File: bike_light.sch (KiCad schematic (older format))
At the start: 0 parts

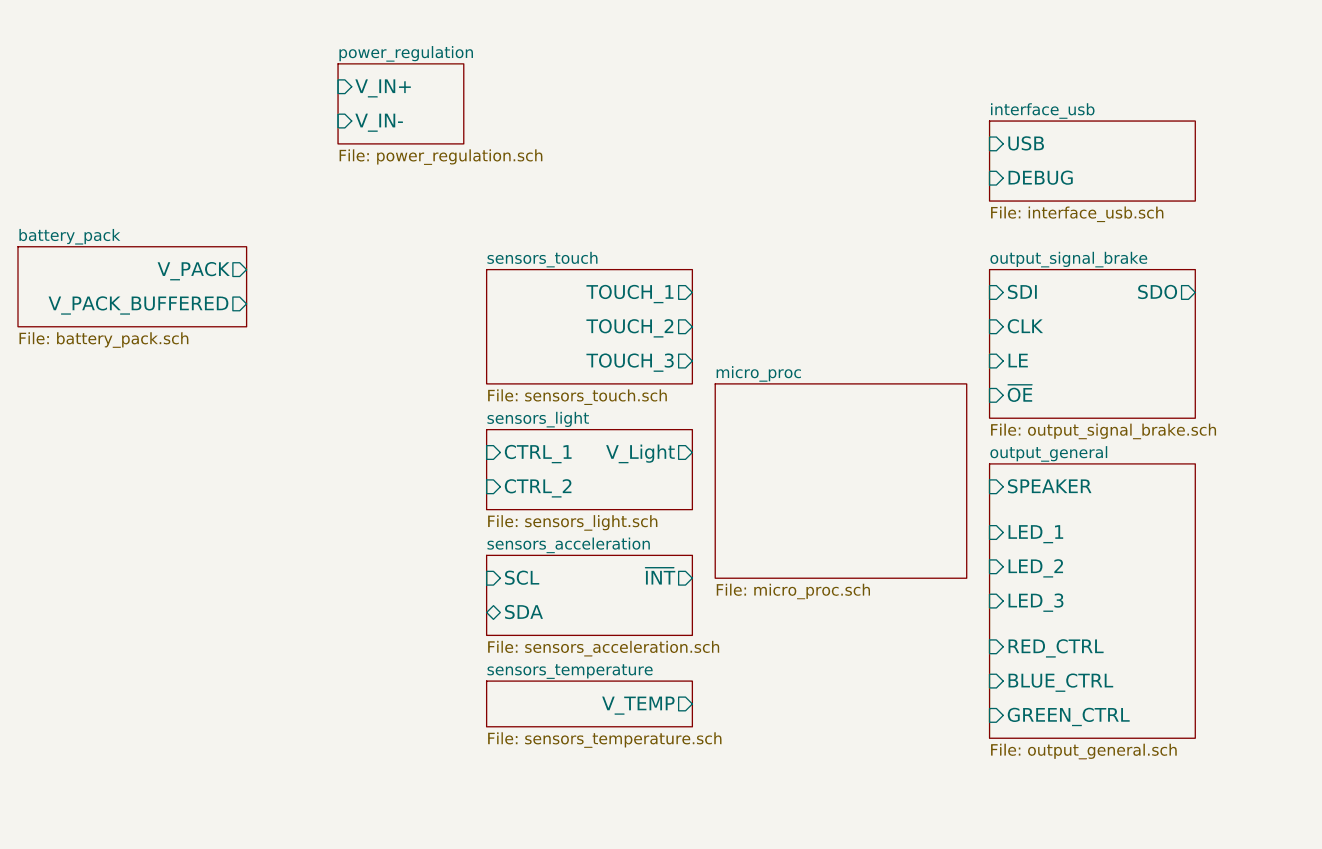
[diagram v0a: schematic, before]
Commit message: random minor thing
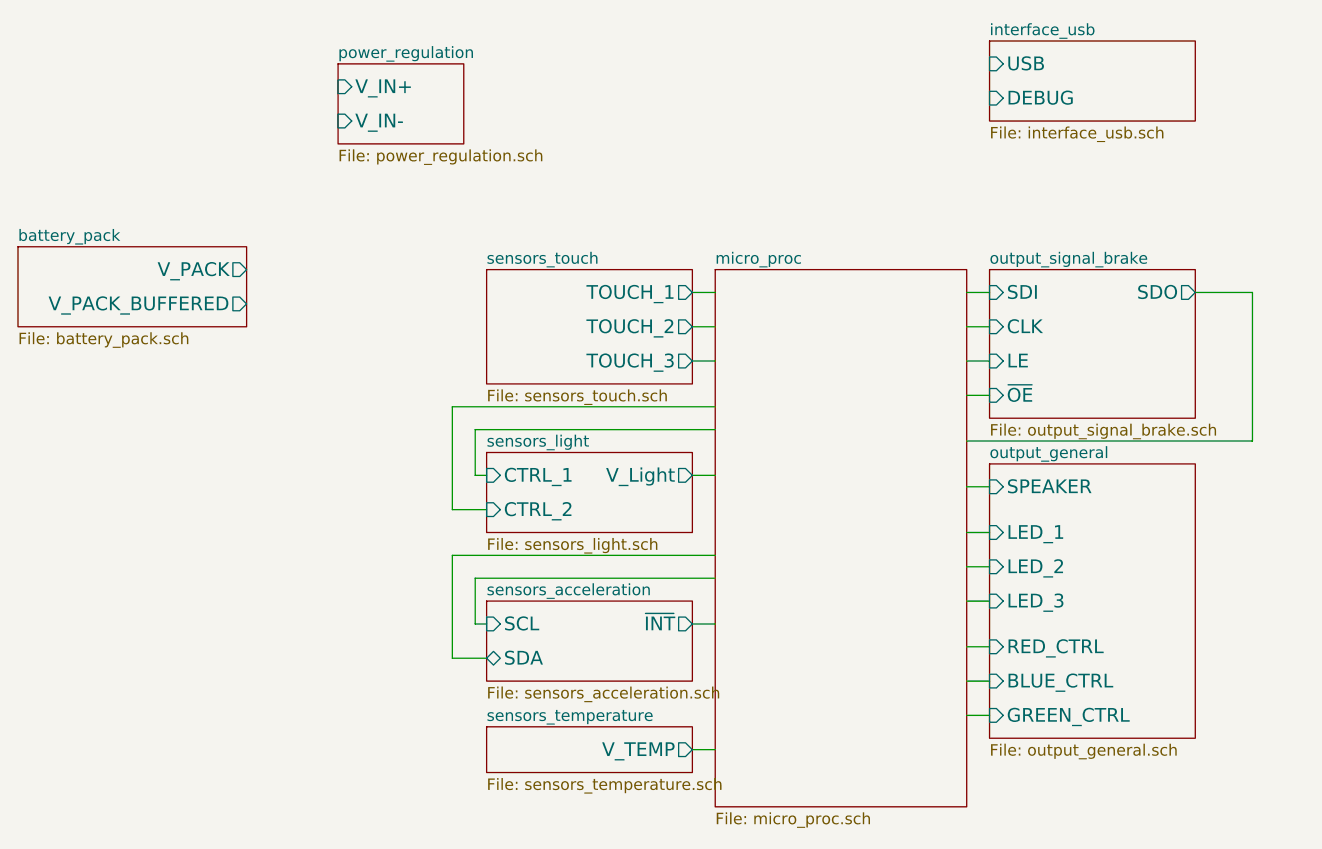
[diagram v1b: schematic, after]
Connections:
- wire segments 0 -> 32
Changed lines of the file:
@@
 Sheet 1 14
 Title "Bike Light"
-Date "12 nov 2013"
+Date "15 nov 2013"
 Rev "1.0"
 Comp ""
@@
 $EndSheet
 $Sheet
-S 5500 2250 1100 850
+S 5500 1750 1100 2350
 U 5224C543
 F0 "micro_proc" 50
@@
 $EndSheet
 $Sheet
-S 6700 1100 900  350
+S 6700 750  900  350
 U 5224C595
 F0 "interface_usb" 50
 F1 "interface_usb.sch" 50
-F2 "USB" I L 6700 1200 60
-F3 "DEBUG" I L 6700 1350 60
+F2 "USB" I L 6700 850 60
+F3 "DEBUG" I L 6700 1000 60
 $EndSheet
 $Sheet
-S 4500 3550 900  200
+S 4500 3750 900  200
 U 527B19B4
 F0 "sensors_temperature" 50
 F1 "sensors_temperature.sch" 50
-F2 "V_TEMP" O R 5400 3650 60
+F2 "V_TEMP" O R 5400 3850 60
 $EndSheet
 $Sheet
-S 4500 2450 900  350
+S 4500 2550 900  350
 U 527B1CA6
 F0 "sensors_light" 50
 F1 "sensors_light.sch" 50
-F2 "V_Light" O R 5400 2550 60
-F3 "CTRL_1" I L 4500 2550 60
-F4 "CTRL_2" I L 4500 2700 60
+F2 "V_Light" O R 5400 2650 60
+F3 "CTRL_1" I L 4500 2650 60
+F4 "CTRL_2" I L 4500 2800 60
 $EndSheet
 $Sheet
-S 4500 3000 900  350
+S 4500 3200 900  350
 U 527C7E4B
 F0 "sensors_acceleration" 50
 F1 "sensors_acceleration.sch" 50
-F2 "SCL" I L 4500 3100 60
-F3 "SDA" B L 4500 3250 60
-F4 "~INT" O R 5400 3100 60
+F2 "SCL" I L 4500 3300 60
+F3 "SDA" B L 4500 3450 60
+F4 "~INT" O R 5400 3300 60
 $EndSheet
 $Sheet
@@
 F8 "GREEN_CTRL" I L 6700 3700 60
 $EndSheet
+Wire Wire Line
+	5400 1850 5500 1850
+Wire Wire Line
+	5400 2000 5500 2000
+Wire Wire Line
+	5400 2150 5500 2150
+Wire Wire Line
+	4500 2650 4450 2650
+Wire Wire Line
+	4450 2650 4450 2450
+Wire Wire Line
+	4450 2450 5500 2450
+Wire Wire Line
+	4500 2800 4350 2800
+Wire Wire Line
+	4350 2800 4350 2350
+Wire Wire Line
+	4350 2350 5500 2350
+Wire Wire Line
+	5400 2650 5500 2650
+Wire Wire Line
+	4500 3300 4450 3300
+Wire Wire Line
+	4450 3300 4450 3100
+Wire Wire Line
+	4450 3100 5500 3100
+Wire Wire Line
+	4500 3450 4350 3450
+Wire Wire Line
+	4350 3450 4350 3000
+Wire Wire Line
+	4350 3000 5500 3000
+Wire Wire Line
+	5400 3300 5500 3300
+Wire Wire Line
+	5400 3850 5500 3850
+Wire Wire Line
+	6600 1850 6700 1850
+Wire Wire Line
+	6700 2000 6600 2000
+Wire Wire Line
+	6700 2150 6600 2150
+Wire Wire Line
+	6700 2300 6600 2300
+Wire Wire Line
+	7600 1850 7850 1850
+Wire Wire Line
+	7850 1850 7850 2500
+Wire Wire Line
+	7850 2500 6600 2500
+Wire Wire Line
+	6700 2700 6600 2700
+Wire Wire Line
+	6700 2900 6600 2900
+Wire Wire Line
+	6700 3050 6600 3050
+Wire Wire Line
+	6700 3200 6600 3200
+Wire Wire Line
+	6700 3400 6600 3400
+Wire Wire Line
+	6700 3550 6600 3550
+Wire Wire Line
+	6700 3700 6600 3700
 $EndSCHEMATC
